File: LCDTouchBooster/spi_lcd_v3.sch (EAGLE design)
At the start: 28 parts, among them IC1 REG1117

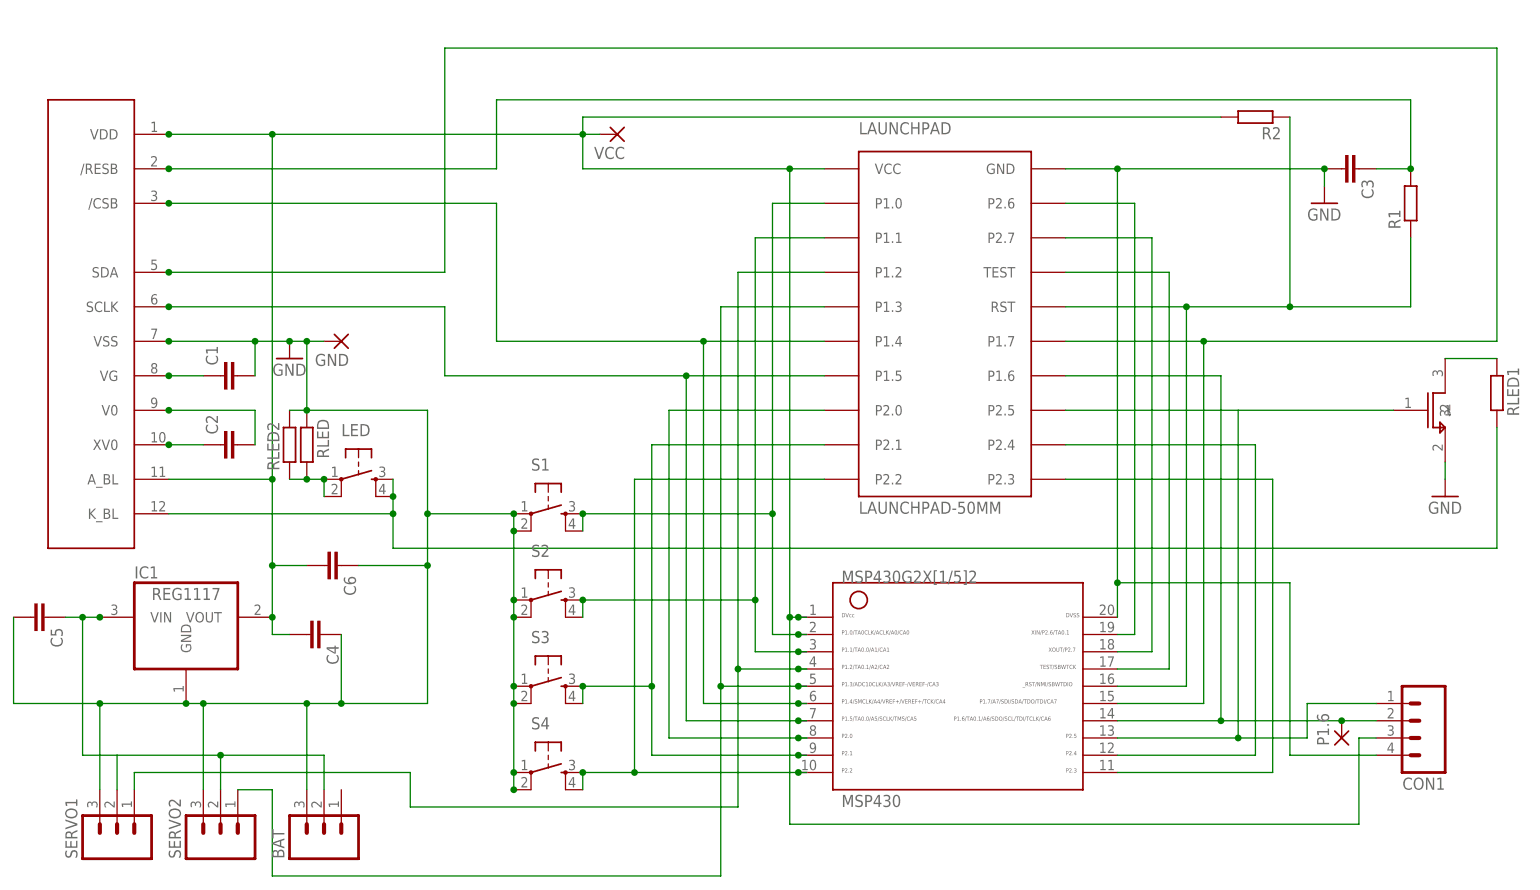
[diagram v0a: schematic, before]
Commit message: Various changes
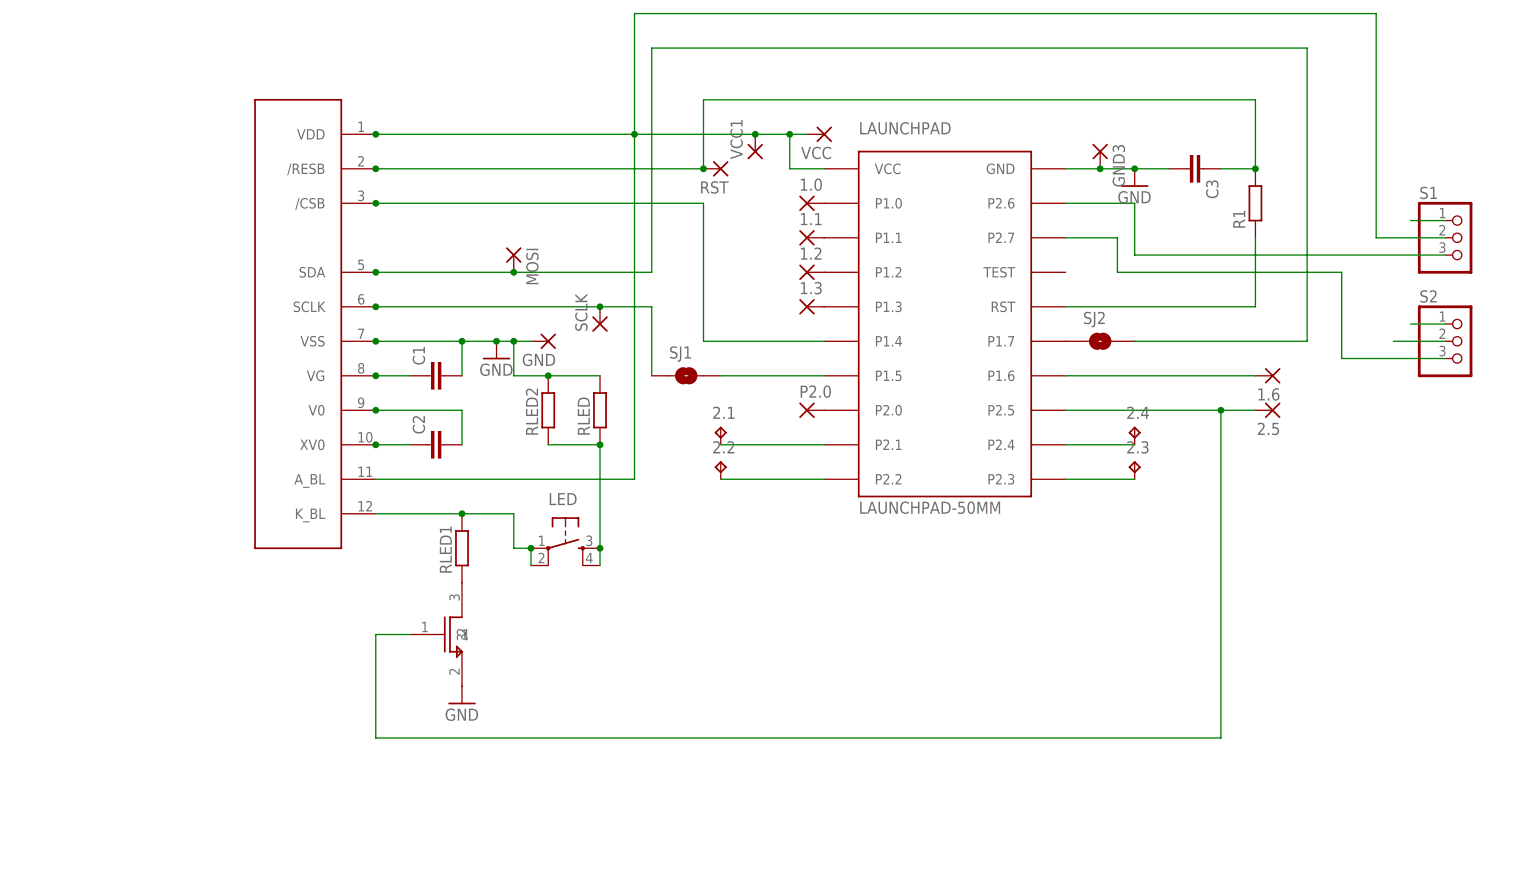
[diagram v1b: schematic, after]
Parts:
- removed BAT, SERVO1, SERVO2: (no value), SparkFun-Connectors:M03PTH
- removed C4, C5, C6: (no value), SparkFun:CAP1206
- removed CON1: (no value), SparkFun-Connectors:M04PTH
- removed IC1: REG1117, burr-brown:REG1117
- removed MSP430: G2X[1/5]2---N20, TI_MSP430_v16:G2X[1/5]2---N20
- removed P1.6: (no value), wirepad:2,15/1,0
- removed R2: (no value), resistor:R-EU_R1206
- removed S3, S4: (no value), SparkFun-Electromechanical:TAC_SWITCHPTH
- added 1.0, 1.1, 1.2, 1.3, 1.6, 2.5, GND3, MOSI, P2.0, RST, SCLK, VCC1: (no value), wirepad:2,15/1,0
- added 2.1, 2.2, 2.3, 2.4: TPTP07R, testpad:TPTP07R
- added SJ1, SJ2: SOLDERJUMPERTRACE, SparkFun-Passives:SOLDERJUMPERTRACE
- RLED2: device resistor:R-EU_0207/10 -> resistor:R-EU_0207/7
- S1, S2: device SparkFun-Electromechanical:TAC_SWITCHPTH -> adafruit:PINHD-1X3
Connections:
- removed net CSB: LAUNCHPAD.P1.4, MSP430.6, U$1./CSB
- removed net KBL: LED.3, LED.4, RLED1.2, U$1.K_BL
- removed net N$22 (its old number): LAUNCHPAD.P2.0, MSP430.8
- removed net P1.0: LAUNCHPAD.P1.0, MSP430.2, S1.3, S1.4
- removed net P1.1: LAUNCHPAD.P1.1, MSP430.3, S2.3, S2.4
- removed net P1.2: LAUNCHPAD.P1.2, MSP430.4, SERVO1.1
- removed net P1.3: LAUNCHPAD.P1.3, MSP430.5, SERVO2.1
- removed net VBAT: BAT.2, C5.1, IC1.VIN, SERVO1.2, SERVO2.2
- removed net VDD: C4.2, C6.2, CON1.3, IC1.VOUT, LAUNCHPAD.VCC, MSP430.1, R2.2, U$1.A_BL, U$1.VDD, VCC.P
- new net N$16: 2.3.TP, LAUNCHPAD.P2.3
- new net N$17: 1.3.P, LAUNCHPAD.P1.3
- new net N$18: LAUNCHPAD.P2.0, P2.0.P
- new net N$19: 1.1.P, LAUNCHPAD.P1.1
- new net N$23: LAUNCHPAD.P2.7, S2.3
- new net N$24: LED.3, LED.4, RLED.1, RLED2.1
- new net N$25: LED.1, LED.2, RLED1.2, U$1.K_BL
- new net N$9: LAUNCHPAD.P1.4, U$1./CSB
- new net VCC: LAUNCHPAD.VCC, S1.2, S2.2, U$1.A_BL, U$1.VDD, VCC.P, VCC1.P
- net GND: now also GND3.P, RLED.2; no longer BAT.3, C4.1, C5.2, C6.1, CON1.4, IC1.GND, MSP430.20, RLED.1, S1.2, S2.2, S3.1, S3.2, S4.1, S4.2, SERVO1.3, SERVO2.3
- net N$10: now also LAUNCHPAD.RST, R1.1; no longer LAUNCHPAD.TEST, MSP430.17
- net N$11: now also 1.6.P, LAUNCHPAD.P1.6; no longer LAUNCHPAD.P2.2, MSP430.10, S4.3, S4.4
- net N$12: now also 1.2.P, LAUNCHPAD.P1.2; no longer CON1.2, LAUNCHPAD.P1.6, MSP430.14, P1.6.P
- net N$13: now also 2.1.TP, LAUNCHPAD.P2.1; no longer CON1.1, LAUNCHPAD.P2.5, LEDSW.1, MSP430.13
- net N$14: now also 2.2.TP, LAUNCHPAD.P2.2; no longer LAUNCHPAD.P2.4, MSP430.12
- net N$15: now also 2.4.TP, LAUNCHPAD.P2.4; no longer LAUNCHPAD.P2.3, MSP430.11
- net N$20: now also LAUNCHPAD.P1.7, SJ2.1; no longer LAUNCHPAD.P2.1, MSP430.9, S3.3, S3.4
- net N$21: now also SJ1.2; no longer MSP430.7, U$1.SCLK
- net N$26: now also LAUNCHPAD.P2.6, S1.3; no longer LED.1, LED.2, RLED.2, RLED2.1
- net N$4: now also 2.5.P, LAUNCHPAD.P2.5, LEDSW.1; no longer LAUNCHPAD.P2.6, MSP430.19
- net N$5: now also RST.P
- net N$6: now also 1.0.P, LAUNCHPAD.P1.0; no longer LAUNCHPAD.P2.7, MSP430.18
- net N$7: now also SCLK.P, SJ1.1, U$1.SCLK; no longer LAUNCHPAD.RST, MSP430.16, R1.1, R2.1
- net N$8: now also MOSI.P, SJ2.2; no longer LAUNCHPAD.P1.7, MSP430.15
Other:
- moved on the sheet: C1, C2, C3, GND, LED, R1, RLED, RLED1, RLED2, VCC
